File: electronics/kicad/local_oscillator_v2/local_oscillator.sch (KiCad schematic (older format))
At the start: 22 parts, among them P1 TestPoint:TestPoint_Pad_1.5x1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, P2 TestPoint:TestPoint_Pad_1.5x1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, P3 TestPoint:TestPoint_Pad_1.5x1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, P4 TestPoint:TestPoint_Pad_1.5x1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, U1 CE3520K3

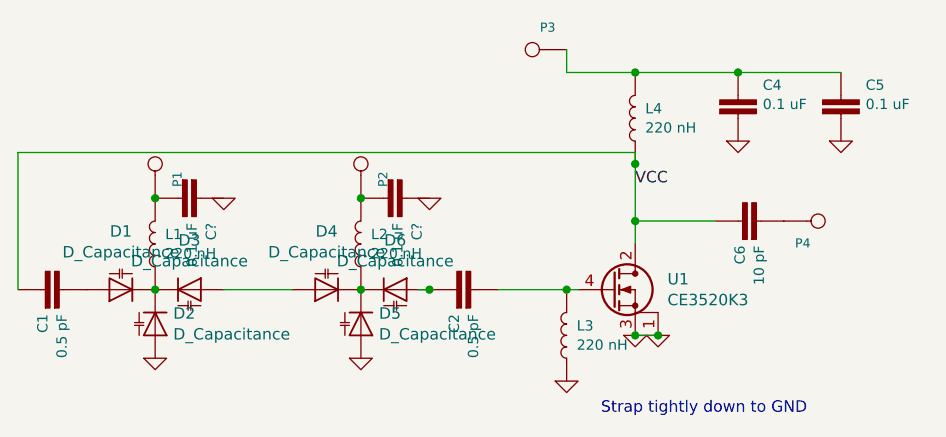
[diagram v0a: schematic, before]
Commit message: Next rev.
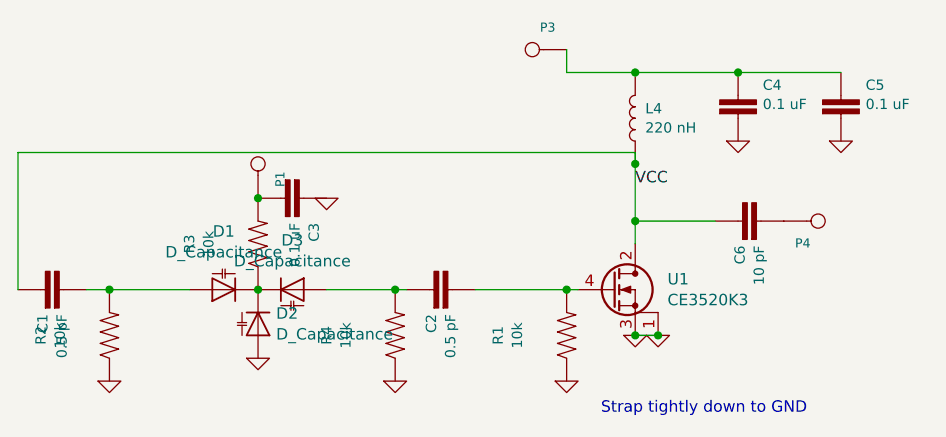
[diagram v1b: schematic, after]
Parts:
- removed C?: 0.1 uF, 0603, symbol SparkFun-Capacitors:4.7UF0603
- removed D4, D5, D6: D_Capacitance, Diode_SMD:D_SOD-523, symbol Device:D_Capacitance
- removed L1, L2, L3: 220 nH, 0402, symbol SparkFun-Coils:INDUCTOR-0402-3.9NH
- removed P2: TestPoint:TestPoint_Pad_1.5x1.5mm, TestPoint:TestPoint_Pad_1.5x1.5mm, symbol conn:CONN_1
- added R1, R2, R3, R4: 10k, 0402, symbol SparkFun-Resistors:RESISTOR0402
- gave numbers to parts that had none: 1
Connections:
- wire segments 15 -> 17
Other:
- moved on the sheet: C2, C3, D1, D2, D3, P1
